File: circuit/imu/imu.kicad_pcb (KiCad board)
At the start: 2 copper layers, 99.5 x 50 mm, 46 parts, among them J1 Batt, J2 DEBUG, J3 Jetson_USB, J4 MIL-14, J5 Jetson, Q1 Q_PMOS_GSD, Q2 Q_PMOS_GSD, U1 OKL-T/6-W12N-C, U2 LPC11U35FHI33/501, U3 PCA9515A, U4 PCA9515A, U5 AQM1602, U6 MPU6500, Y1 12M

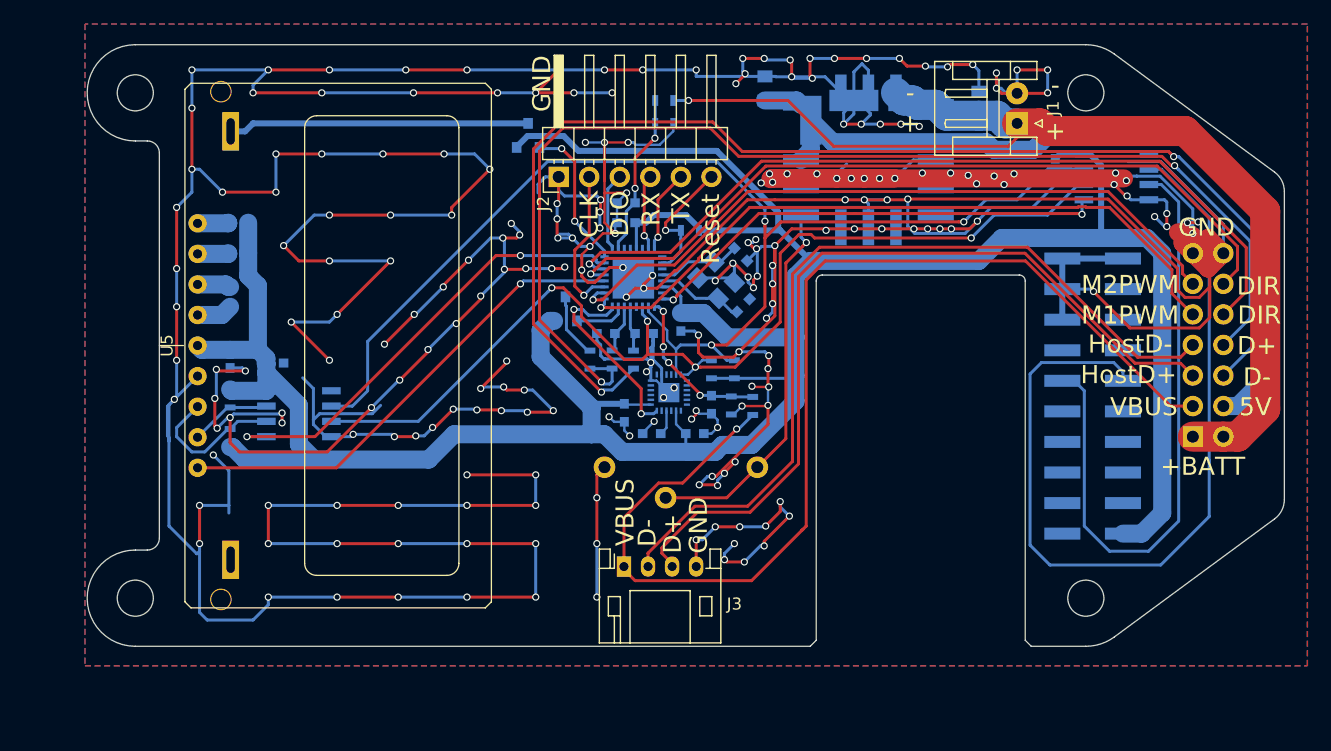
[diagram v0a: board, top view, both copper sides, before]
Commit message: update circuits
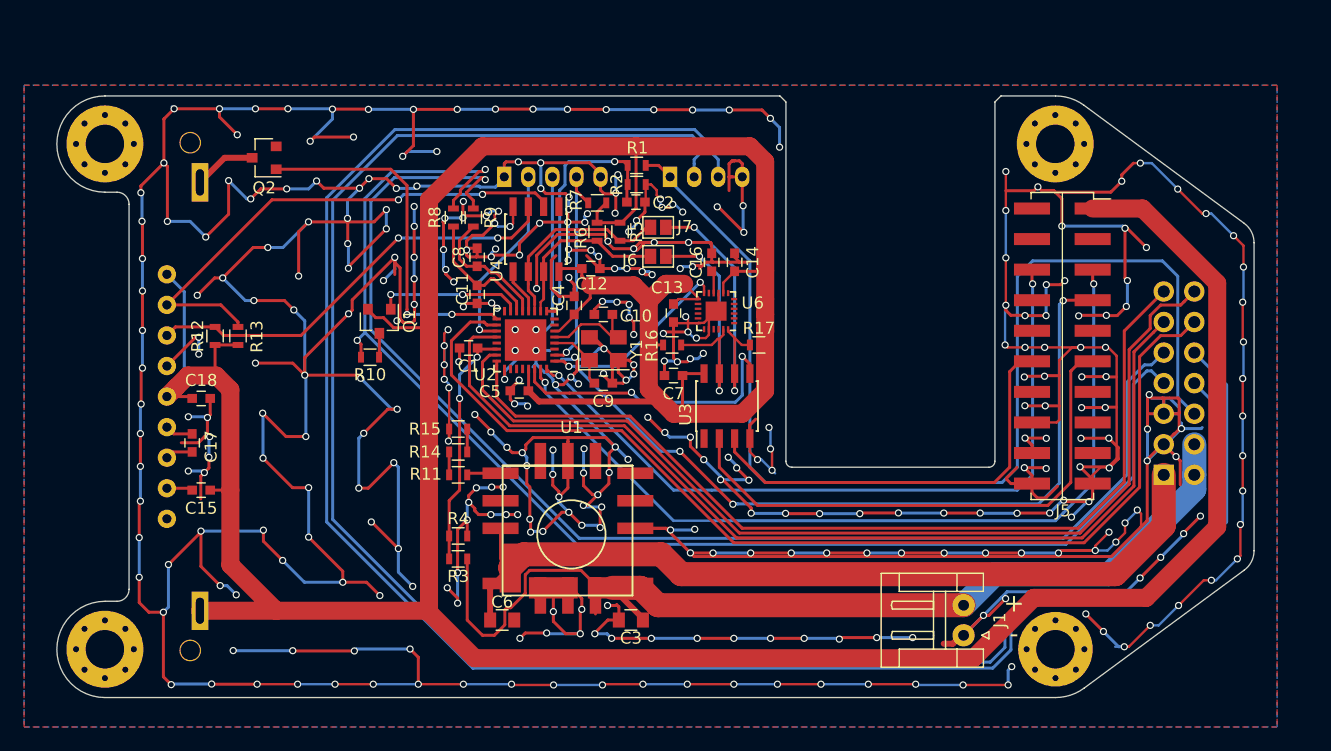
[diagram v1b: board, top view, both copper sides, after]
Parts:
- removed RV1: 2k, Potentiometers:Potentiometer_Trimmer_Bourns_3006P
- added J6: GS2, Connectors:GS2, F.Cu at (146.7, 98.0)
- added J7: GS2, Connectors:GS2, F.Cu at (146.7, 95.6)
- added R14: 330, Resistors_SMD:R_0603, F.Cu at (130.1, 114.3)
- added R15: 10, Resistors_SMD:R_0603, F.Cu at (130.1, 112.4)
- added R16: 4.7k, Resistors_SMD:R_0603, F.Cu at (147.9, 105.4)
- added R17: 4.7k, Resistors_SMD:R_0603, F.Cu at (155.1, 105.4)
- added REF**: MountingHole_3.2mm_M3_Pad_Via, Mounting_Holes:MountingHole_3.2mm_M3_Pad_Via, F.Cu at (179.7, 130.7)
- added REF**: MountingHole_3.2mm_M3_Pad_Via, Mounting_Holes:MountingHole_3.2mm_M3_Pad_Via, F.Cu at (179.7, 88.7)
- added REF**: MountingHole_3.2mm_M3_Pad_Via, Mounting_Holes:MountingHole_3.2mm_M3_Pad_Via, F.Cu at (100.7, 130.7)
- added REF**: MountingHole_3.2mm_M3_Pad_Via, Mounting_Holes:MountingHole_3.2mm_M3_Pad_Via, F.Cu at (100.7, 88.7)
- C1, C10, C11, C12, C13, C14, C15, C16, C17, C18, C2, C3, C4, C5, C6, C7, C8, C9, J5, Q1, R1, R10, R12, R13, R2, R3, R4, R7, R8, R9, U1, U2, U3, U4, U6: moved to F.Cu
- J2: value DEBUG -> Debug; footprint Pin_Headers:Pin_Header_Angled_1x06_Pitch2.54mm -> Connectors_JST:JST_PH_S5B-PH-K_05x2.00mm_Angled; moved to B.Cu
- J3, U5: moved to B.Cu
- Q2: value Q_PMOS_GSD -> Q_NMOS_GSD; moved to F.Cu
- R11: value R -> 1k; moved to F.Cu
- R5, R6: value 2k -> 4.7k; moved to F.Cu
- Y1: footprint Oscillators:Oscillator_SMD_SeikoEpson_SG8002CE-4pin_3.2x2.5mm -> Crystals:Crystal_SMD_SeikoEpson_FA238V-4pin_3.2x2.5mm; moved to F.Cu
- moved C3 51.7 mm to (144.4, 128.3), turned to 180 degrees
- moved C6 49.3 mm to (133.7, 128.3), turned to 0 degrees
- moved J1 42.8 mm to (172.1, 129.5)
- moved R3 41.8 mm to (130.1, 123.2)
- moved U1 40.3 mm to (139.5, 121.2)
- moved R4 38.3 mm to (130.1, 121.3)
- moved U3 37.6 mm to (152.4, 110.5), turned to 90 degrees
- moved C7 36.1 mm to (148.0, 108.0), turned to 180 degrees
- moved J3 32.6 mm to (147.7, 91.4)
- moved R11 27.8 mm to (130.1, 116.2), turned to 0 degrees
- moved C12 27.4 mm to (141.1, 99.1)
- moved U4 24.5 mm to (136.5, 96.6), turned to 270 degrees
- moved R1 22.2 mm to (144.9, 90.5), turned to 180 degrees
- moved Q2 22.0 mm to (114.0, 89.9), turned to 180 degrees
- moved R2 20.0 mm to (144.9, 92.1), turned to 0 degrees
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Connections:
- C1 pad 1: /ADC5 -> /ADC1
- J1 pad 1: +BATT -> GND
- J1 pad 2: GND -> +BATT
- J2 pad 4: /RXD -> /~MCU_RESET
- J2 pad 5: /TXD -> GND
- J4 pad 1: +BATT -> +5V
- J4 pad 10: /ADC1 -> /HostD+
- J4 pad 11: /M2PWM -> /M1PWM
- J4 pad 12: /ADC0 -> /M1DIR
- J4 pad 13: GND -> /ADC3/PWM10
- J4 pad 14: GND -> /ADC2/PWM9
- J4 pad 3: VBUS -> GND
- J4 pad 4: +5V -> +BATT
- J4 pad 5: /HostD+ -> GND
- J4 pad 6: /D- -> VBUS
- J4 pad 7: /HostD- -> /D+
- J4 pad 8: /D+ -> /HostD-
- J4 pad 9: /M1PWM -> /D-
- J5 pad 5: (no net) -> /JETSON_TX1
- J5 pad 6: (no net) -> /JETSON_RX1
- J5 pad 7: (no net) -> /IMU_INT
- Q2 pad 1: /ADC3/PWM10 -> /LCD_CONTRAST
- Q2 pad 2: +3V3 -> GND
- R11 pad 1: +3V3 -> Net-(R11-Pad1)
- R3 pad 2: /ADC5 -> /ADC1
- R4 pad 1: /ADC5 -> /ADC1
- R5 pad 2: /SDA -> /MCU_SDA
- R6 pad 2: /SCL -> /MCU_SCL
- U1 pad 6: Net-(RV1-Pad1) -> Net-(R11-Pad2)
- U2 pad 1: (no net) -> /IMU_INT
- U2 pad 10: /SCL -> /MCU_SCL
- U2 pad 11: /SDA -> /MCU_SDA
- U2 pad 12: (no net) -> /LCD_EN
- U2 pad 16: /IMU_INT -> (no net)
- U2 pad 17: /M1PWM -> /LCD_CONTRAST
- U2 pad 18: /M2PWM -> /M1DIR
- U2 pad 20: /~LCD_RESET -> /M1PWM
- U2 pad 21: /ADC0 -> (no net)
- U2 pad 26: /ADC5 -> (no net)
- U2 pad 30: (no net) -> /JETSON_EN
- U2 pad 31: /RXD -> /JETSON_TX1
- U2 pad 32: /TXD -> /JETSON_RX1
- U2 pad 8: /JETSON_EN -> (no net)
- U3 pad 6: /SDA -> /IMU_SDA
- U3 pad 7: /SCL -> /IMU_SCL
- U4 pad 2: /SCL -> Net-(R13-Pad2)
- U4 pad 3: /SDA -> Net-(R12-Pad2)
- U4 pad 5: /ADC2/PWM9 -> /LCD_EN
- U4 pad 6: Net-(R12-Pad2) -> /MCU_SDA
- U4 pad 7: Net-(R13-Pad2) -> /MCU_SCL
- U5 pad 1: Net-(R11-Pad2) -> (no net)
- U5 pad 10: Net-(Q2-Pad3) -> +3V3
- U5 pad 11: GND -> Net-(Q2-Pad3)
- U5 pad 9: /~LCD_RESET -> +3V3
- U6 pad 23: /SCL -> /IMU_SCL
- U6 pad 24: /SDA -> /IMU_SDA
- U6 pad 9: (no net) -> GND
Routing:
- net GND: track 936.4 -> 1192.8 mm, vias 226 -> 372
- net /SCL: track 104.0 -> 0.00 mm, vias 3 -> 0
- net /HostD+: track 69.5 -> 165.7 mm
- net /HostD-: track 70.2 -> 159.6 mm
- net /M1DIR: track 0.00 -> 88.8 mm
- net +3V3: track 247.8 -> 336.5 mm
- net /SDA: track 87.8 -> 0.00 mm, vias 4 -> 0
- net /JETSON_TX1: track 0.00 -> 71.2 mm, vias 0 -> 2
- net /ADC3/PWM10: track 12.4 -> 78.5 mm, vias 2 -> 0
- net /ADC0: track 65.0 -> 0.00 mm, vias 1 -> 0
- net /IMU_INT: track 16.2 -> 79.7 mm, vias 2 -> 5
- net /JETSON_RX1: track 0.00 -> 62.2 mm, vias 0 -> 2
- net /M2PWM: track 58.5 -> 0.00 mm, vias 1 -> 0
- net /ADC1: track 68.9 -> 20.1 mm, vias 1 -> 2
- net /ADC2/PWM9: track 38.0 -> 83.3 mm, vias 2 -> 0
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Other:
- outline, holes or cut-outs redrawn
- board text added: "H+"
- board text added: "H-"
- board text added: "SWCLK"
- board text added: "SWDIO"
- board text added: "VB"
- board text added: "nReset"
- board text removed: "CLK"
- board text removed: "DIO"
- board text removed: "HostD+"
- board text removed: "HostD-"
- board text removed: "RX"
- board text removed: "Reset"
- board text removed: "TX"
